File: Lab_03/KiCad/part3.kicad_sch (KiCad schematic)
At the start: 14 parts, among them U3 LM741, U5 LM339

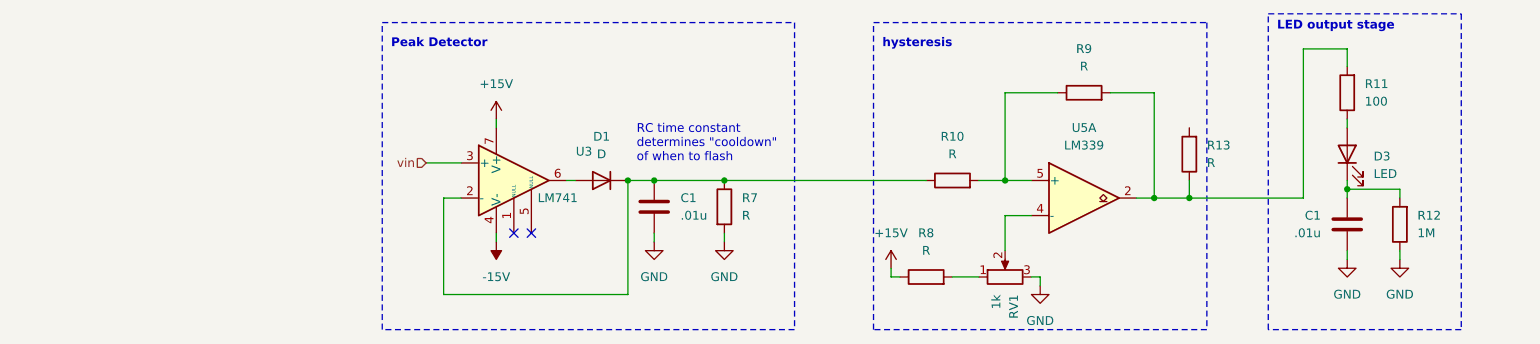
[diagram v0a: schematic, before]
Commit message: markey push
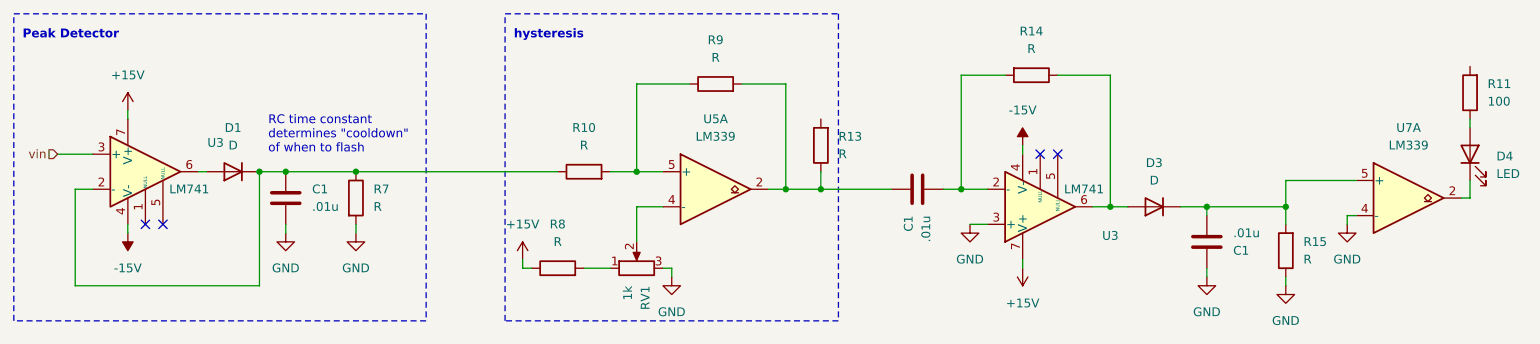
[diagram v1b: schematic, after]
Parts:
- removed C1: .01u, symbol Device:C
- removed D3: LED, symbol Device:LED
- removed R12: 1M, symbol Device:R
- added C1 (x2): .01u, symbol Device:C
- added D3: D, symbol Device:D
- added D4: LED, symbol Device:LED
- added R14, R15: R, symbol Device:R
- added U3: LM741, symbol Amplifier_Operational:LM741
- added U7: LM339, symbol Comparator:LM339
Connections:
- net +15V: now also U3.7 (V+)
- net -15V: now also U3.4 (V-)
- net GND: now also C1.1, R15.1, U3.3 (+), U7.4 (-)
- net at R13.1, R9.2, U5.2: now also C1.1; no longer R11.2
- net at R11.1: now also D4.2 (A)
- new net: C1.2, R14.2, U3.2 (-)
- new net: D3.2 (A), R14.1, U3.6
- new net: D4.1 (K), U7.2
- new net: C1.2, D3.1 (K), R15.2, U7.5 (+)
- no-connect marks 2 -> 4
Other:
- note removed: "LED output stage"
- moved on the sheet: C1, D1, R10, R13, R7, R8, R9, RV1, U3, U5A
